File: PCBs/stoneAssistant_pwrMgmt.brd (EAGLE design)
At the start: 65.3 x 58.2 mm, 58 parts, among them IC1 TINY2313-*S*, IC2 CNY17, IC3 CPC1976Y, IC4 CPC1976Y, J4 DISPLAY, T4 IRLML6402, T7 IRLML6402, X3 BTN_ON

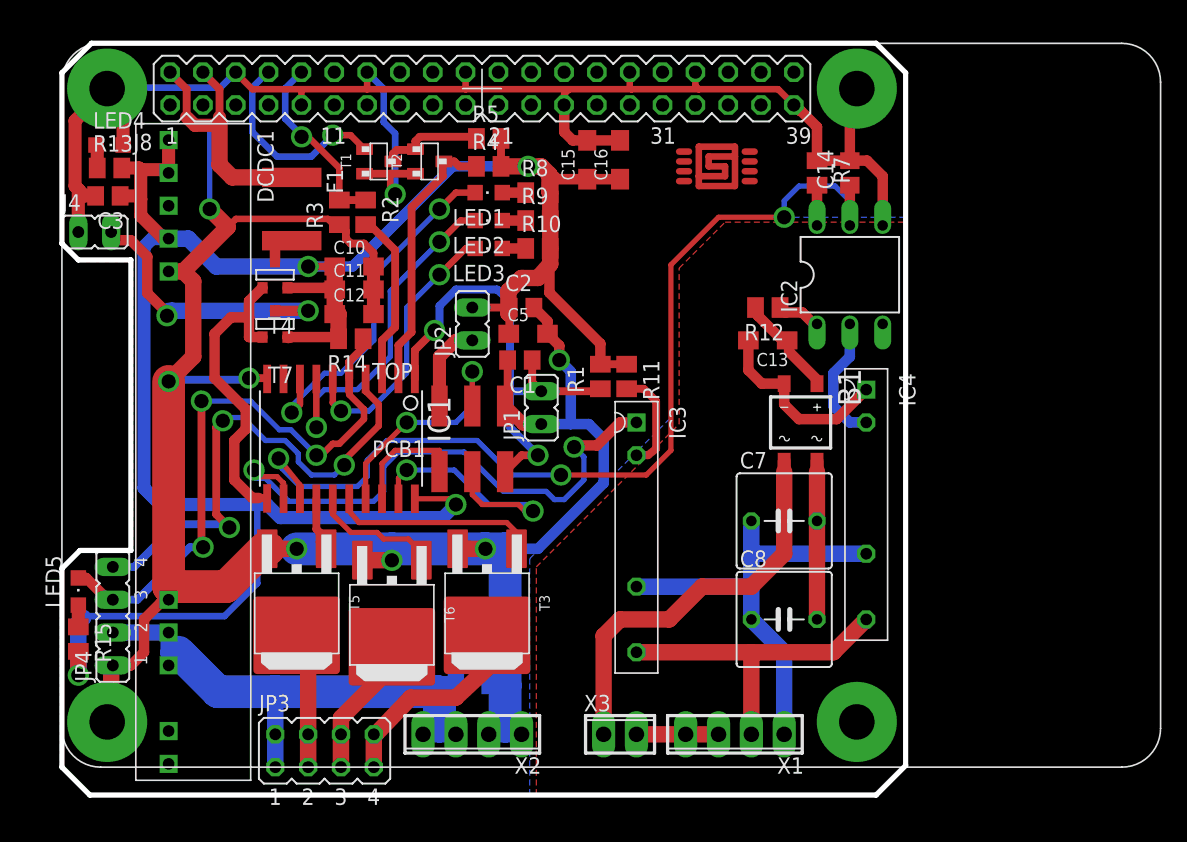
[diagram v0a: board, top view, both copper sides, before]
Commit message: final power management pcb
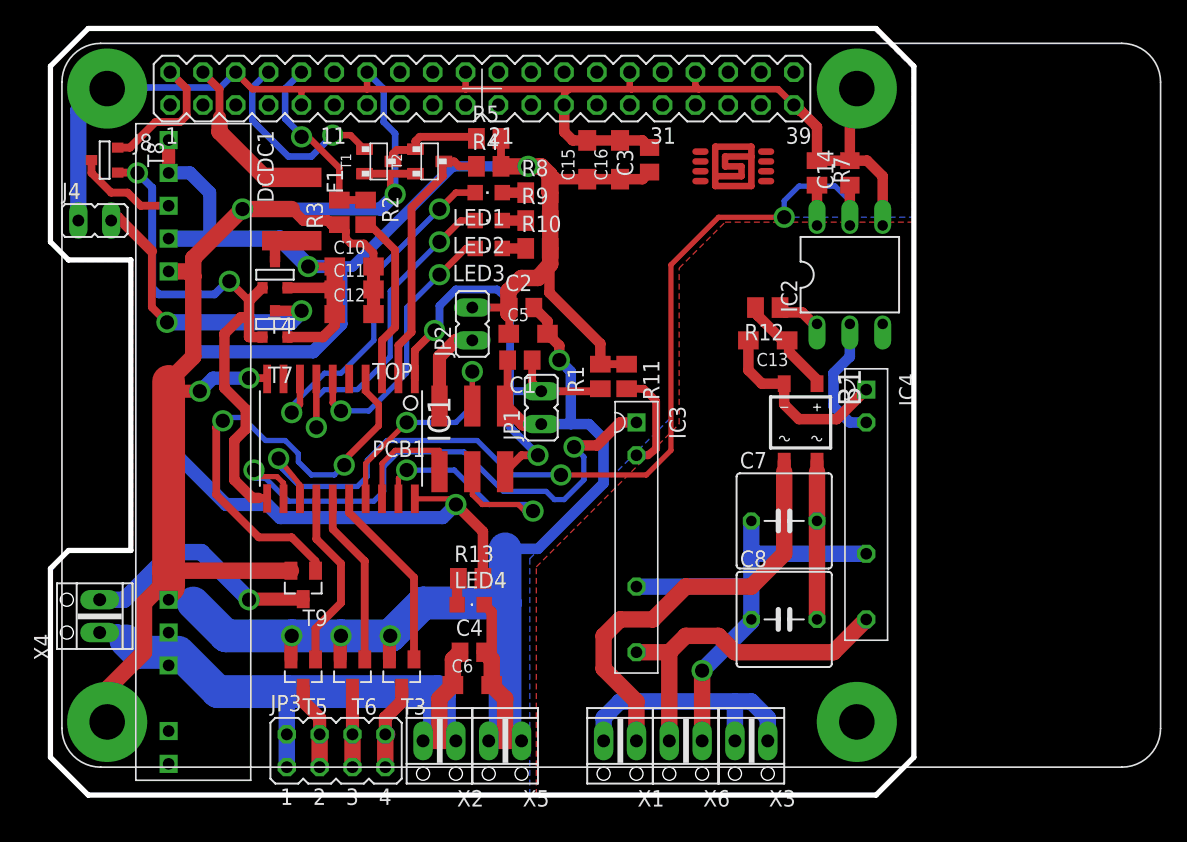
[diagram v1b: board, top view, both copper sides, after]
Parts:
- removed JP4: FAN, jumper:JP4
- removed LED5: (no value), led:CHIPLED_0805
- removed R14: 18k, rcl:M0805
- removed R15: 270R, rcl:M0805
- added T8: IRLML6402, IRLML6402:SOT-23
- added T9: IRLML2502, nxs_transistor:SOT-23
- added X4: FAN, nxs_con-misc:2_2.54MM
- added X5: GND, nxs_con-misc:2_2.54MM
- added X6: L, nxs_con-misc:2_2.54MM
- T3, T5, T6: value (none) -> IRLML2502; device we-transistor:DPAK_TO252 -> nxs_transistor:SOT-23
- X1: value (none) -> BTN_ON; device con-phoenix-254:4POL254 -> nxs_con-misc:2_2.54MM
- X2: value (none) -> +12V; device con-phoenix-254:4POL254 -> nxs_con-misc:2_2.54MM
- X3: value BTN_ON -> N; device con-phoenix-254:2POL254 -> nxs_con-misc:2_2.54MM
- moved LED4 45.2 mm to (31.6, 12.6)
- moved R13 42.3 mm to (31.6, 14.6)
- moved C3 42.0 mm to (45.5, 47.0), turned to 90 degrees
- moved X3 10.2 mm to (53.3, 2.03), turned to 180 degrees
- moved X1 8.90 mm to (43.2, 2.03)
- moved T3 8.57 mm to (26.3, 7.24), turned to 180 degrees
- moved T6 5.49 mm to (22.5, 7.24), turned to 180 degrees
- moved T5 5.48 mm to (18.7, 7.24), turned to 180 degrees
- moved X2 2.59 mm to (29.2, 2.03)
- moved JP3 0.89 mm to (21.2, 1.27)
- moved J4 0.89 mm to (2.54, 42.3)
- flipped C4 to the top, turned to 0 degrees
- flipped C6 to the top, turned to 0 degrees
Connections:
- removed net FAN_SIGNAL: IC1.5, JP4.3, LED5.C, R14.1
- new net 5V_FB: DCDC1.3, T8.3
- new net N$32: PCB1.2, T8.2
- net +12V: now also X2.1, X2.2, X4.1; no longer JP4.2, X2.3, X2.4
- net +5V: no longer R14.2, R15.2
- net FAN_PWM: now also T9.1; no longer JP4.4
- net GND: now also T3.2, T5.2, T6.2, T9.2, X5.1, X5.2; no longer JP4.1, T3.3, T5.3, T6.3, X2.1, X2.2
- net N$10: now also X6.2; no longer X1.2
- net N$11: now also X6.1; no longer X1.1
- net N$12: now also X1.2, X3.1; no longer X1.3, X1.4
- net N$16: now also X1.1; no longer X3.1
- net N$21: now also T5.3; no longer T5.2
- net N$22: now also T6.3; no longer T6.2
- net N$23: now also T3.3; no longer T3.2
- net N$25: now also T9.3, X4.2; no longer LED5.A, R15.1
- net RPI_5V: no longer PCB1.2
- net RPI_SUPPLY: now also T8.1
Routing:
- net FAN_SIGNAL: track 46.0 -> 0.00 mm, vias 3 -> 0
- net +5V: track 179.9 -> 158.7 mm, vias 4 -> 3
- net GND: track 297.1 -> 318.0 mm
- net RPI_SUPPLY: track 24.3 -> 42.9 mm, vias 0 -> 2
- net N$25: track 1.68 -> 18.8 mm, vias 0 -> 1
- net N$12: track 6.35 -> 20.4 mm
- net N$23: track 17.2 -> 6.81 mm
- net N$32: track 0.00 -> 10.2 mm
- net PWM_G: track 4.18 -> 14.0 mm
- net RPI_5V: track 20.5 -> 12.2 mm
- net +12V: track 45.3 -> 53.5 mm
- net 5V_FB: track 0.00 -> 8.01 mm
- net N$22: track 12.2 -> 6.14 mm
- net N$21: track 11.1 -> 6.67 mm
- net PWM_R: track 9.90 -> 13.5 mm
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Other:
- board size 65.3 x 58.2 mm -> 66.8 x 59.3 mm
- board text added: "+"
- board text added: "-"
- board text added: "14.6.2018"
- board text added: "B1"
- board text added: "C1"
- board text added: "C10"
- board text added: "C11"
- board text added: "C12"
- board text added: "C13"
- board text added: "C14"
- board text added: "C15"
- board text added: "C16"
- board text added: "C2"
- board text added: "C3"
- board text added: "C4"
- board text added: "C5"
- board text added: "C6"
- board text added: "C7"
- board text added: "C8"
- board text added: "DCDC1"
- board text added: "F1"
- board text added: "IC1"
- board text added: "IC2"
- board text added: "IC3"
- board text added: "IC4"
- board text added: "ICSP"
- board text added: "JP3"
- board text added: "LCD"
- board text added: "LED1"
- board text added: "LED2"
- board text added: "LED3"
- board text added: "LED4"
- board text added: "MAINS"
- board text added: "R1"
- board text added: "R10"
- board text added: "R11"
- board text added: "R12"
- board text added: "R13"
- board text added: "R2"
- board text added: "R3"
- board text added: "R4"
- board text added: "R5"
- board text added: "R7"
- board text added: "R8"
- board text added: "R9"
- board text added: "RST"
- board text added: "SUPPLY"
- board text added: "T1"
- board text added: "T2"
- board text added: "T3"
- board text added: "T4"
- board text added: "T5"
- board text added: "T6"
- board text added: "T7"
- board text added: "T8"
- board text added: "T9"
- board text added: "TARGET"
- board text added: "VOLTAGE"
- board text added: "X1"
- board text added: "X2"
- board text added: "X3"
- board text added: "X4"
- board text added: "X5"
- board text added: "X6"
- board text added: "by everyone"
- board text added: "free to use"
- board text added: "github.com/stonetronics"
- board text added: "pwr & pwm"
- board text removed: "pwr&pwm"
